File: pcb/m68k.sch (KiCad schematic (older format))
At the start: 120 parts, among them J1 USB_B_Micro, J2 Mini-DIN-6, J4 DB15_Male_HighDensity, J5 FTSH-105-01-L-DV-K, J6 FTSH-105-01-L-DV-K, J7 FTSH-105-01-L-DV-K, J8 Micro_SD_Card, U1 93LC56, U10 25LCxxx, U11 TXB0108DQSR, U12 TXB0108DQSR, U13 iCE40-HX4K-TQ144, U14 ADV7125KSTZ50, U15 74LVC1G17, U16 LD1117S33TR_SOT223, U17 LD1117S12TR_SOT223, U18 ATL431BQDBZR, U2 68000D, U3 FT2232H, U4 TXB0108DQSR, U5 TXB0108DQSR, U6 TXB0108DQSR, U7 SN74LVC8T245PWR, U8 SN74LVC8T245PWR, U9 AS6C1616, X1 ASV-12.000MHz

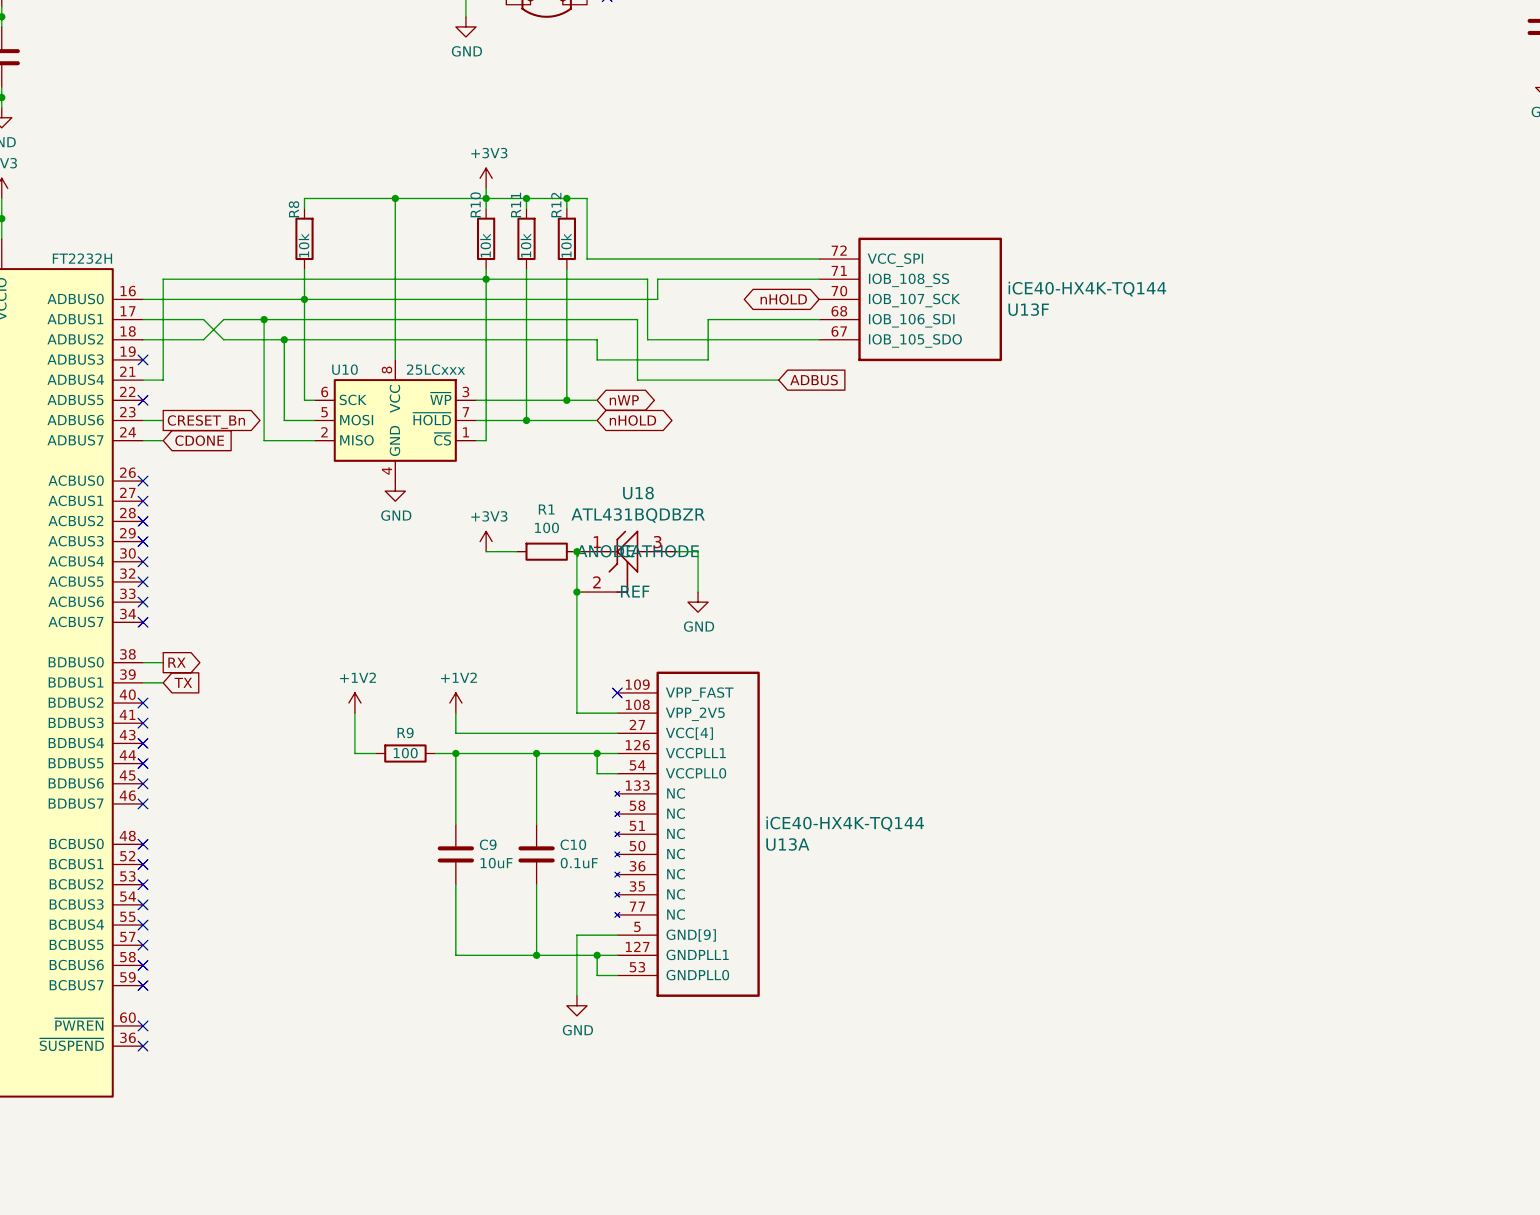
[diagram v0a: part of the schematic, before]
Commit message: clean up pins
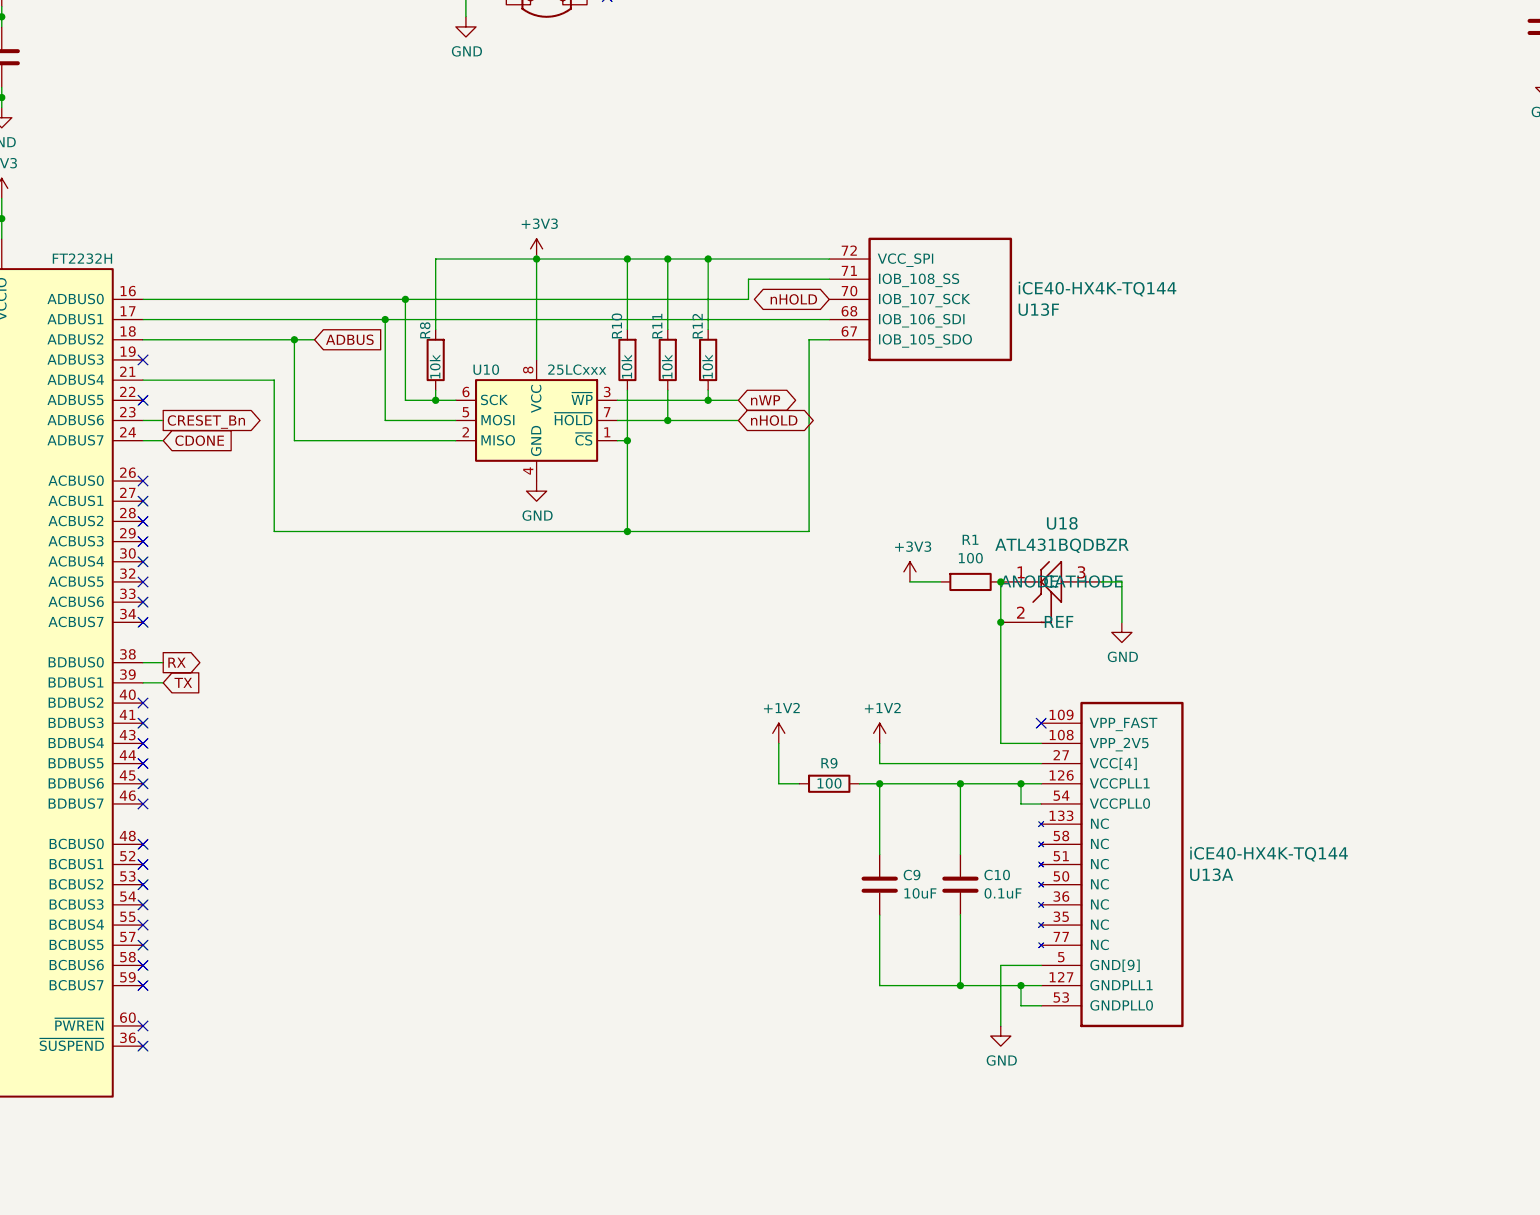
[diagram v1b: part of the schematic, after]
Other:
- moved on the sheet: C10, C9, R1, R10, R11, R12, R8, R9, U10, U13A, U13F, U18
